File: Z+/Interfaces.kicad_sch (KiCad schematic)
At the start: 13 parts, among them J1 200528-0100, J2 Conn_01x04_MountingPin, J3 USB4110GFA, J4 BG301-06-X-XXXX-X-X_REVC, J5 BG301-06-X-XXXX-X-X_REVC, U1 USBLC6-2P6, U10 USBLC6-2P6

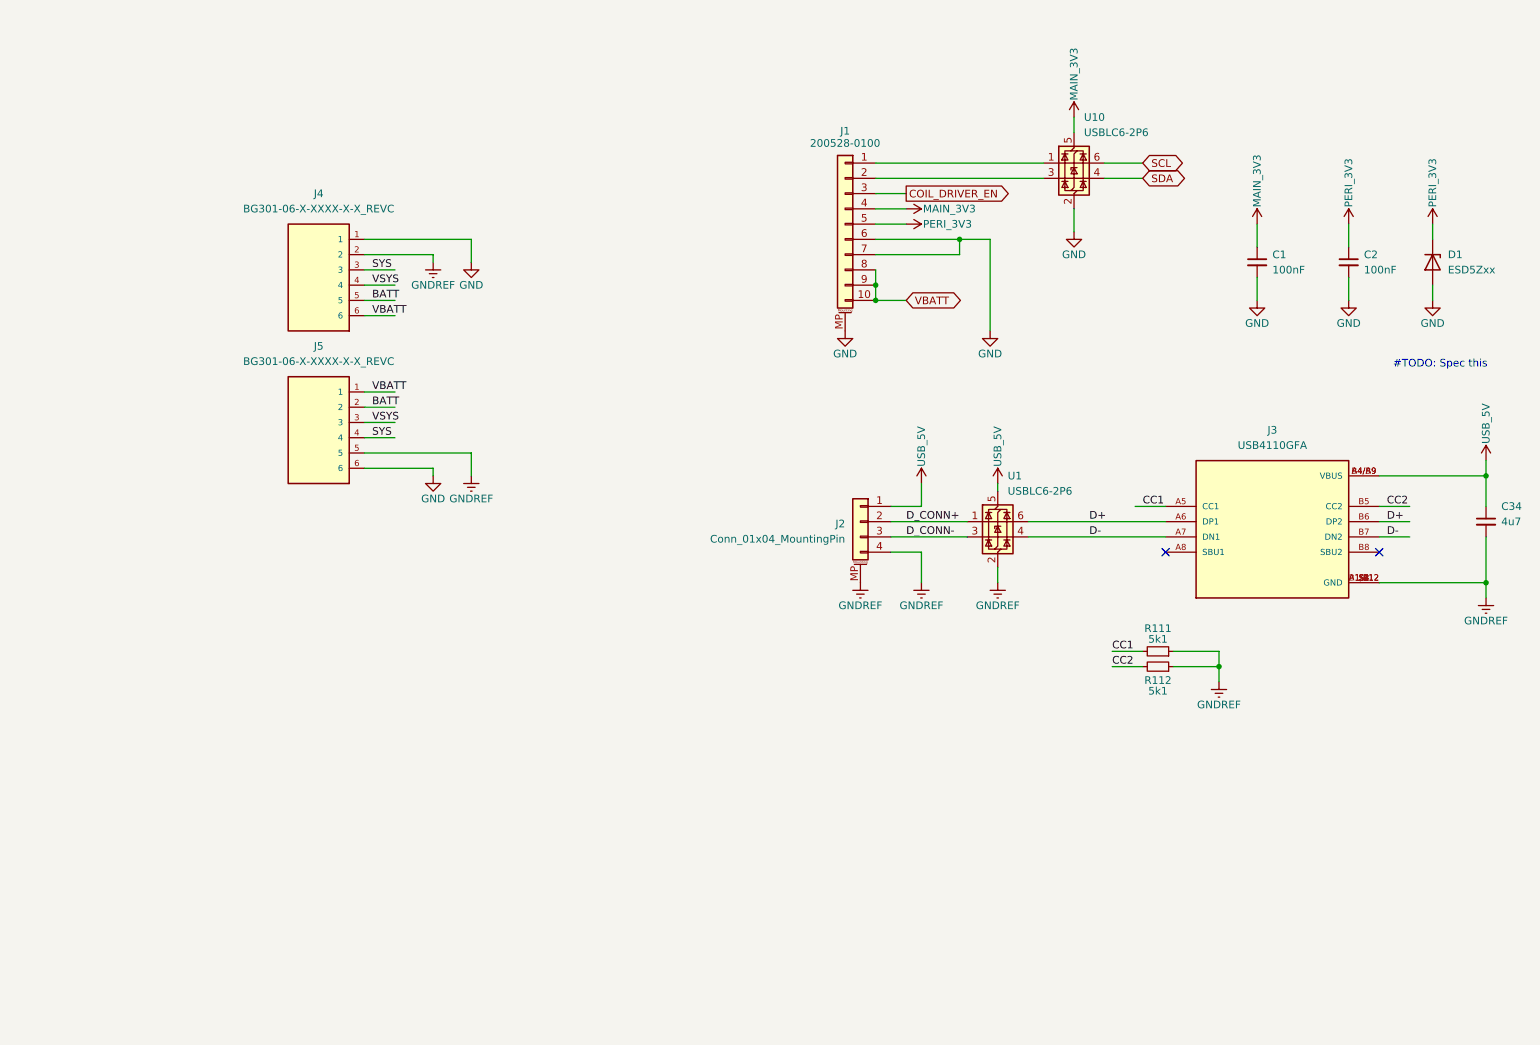
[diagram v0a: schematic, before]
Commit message: More layout work
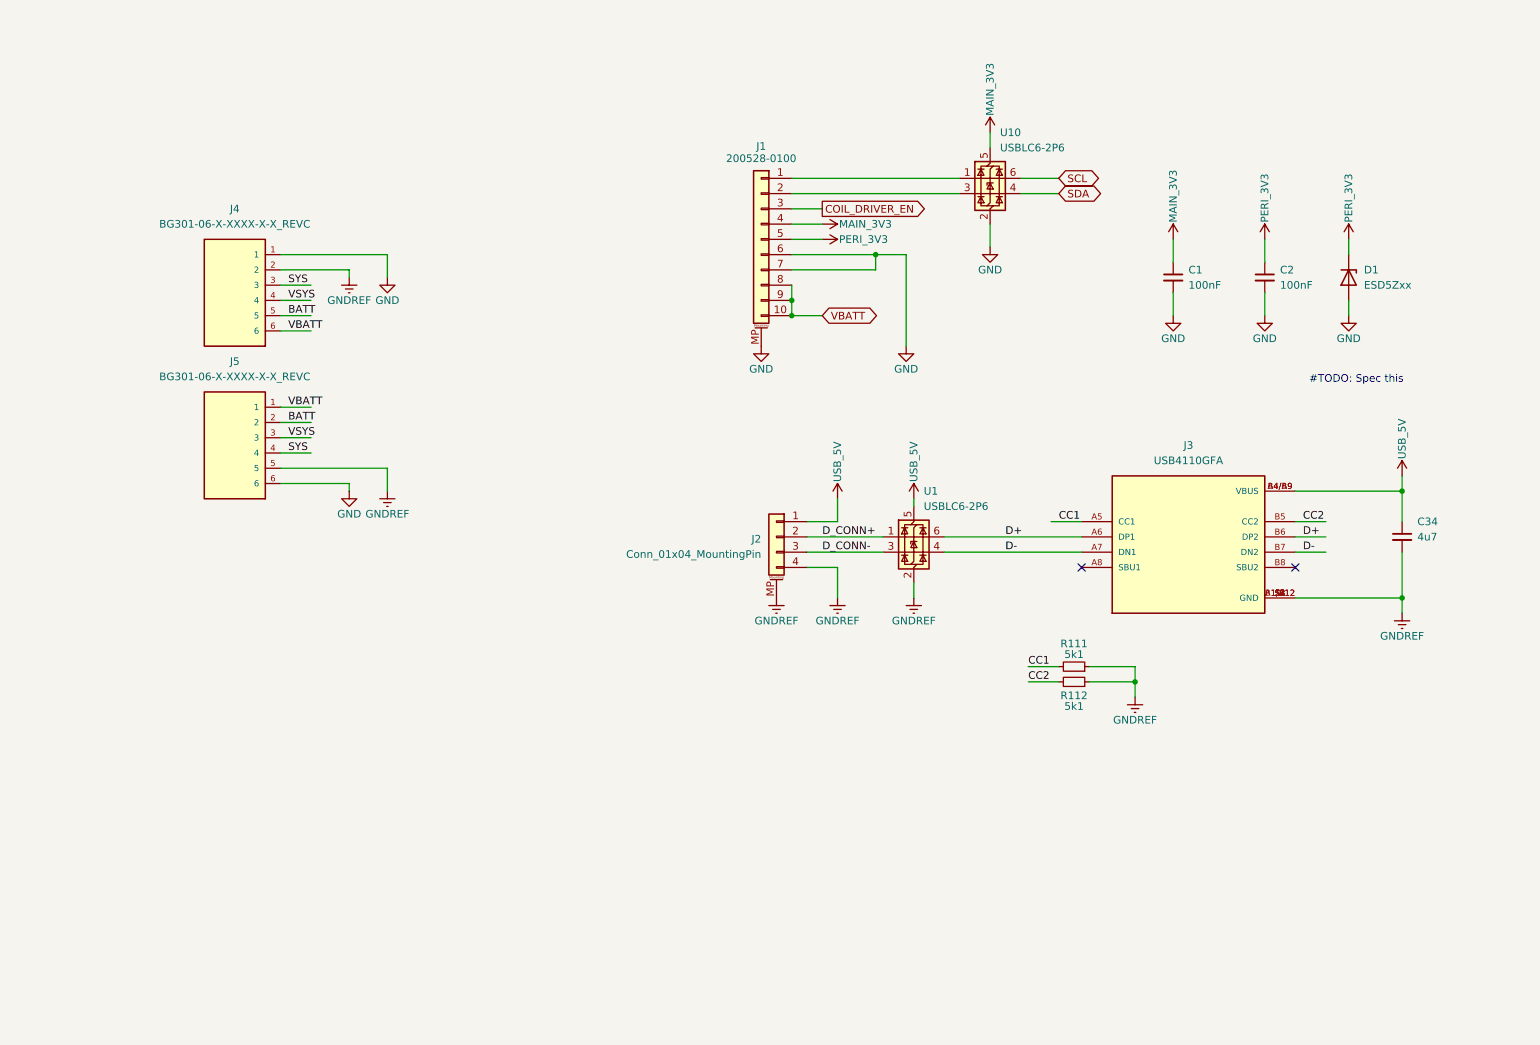
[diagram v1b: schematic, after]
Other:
- moved on the sheet: C1, C2, C34, D1, J1, J2, J3, J4, J5, R111, R112, U1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

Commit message: Finished layout v1
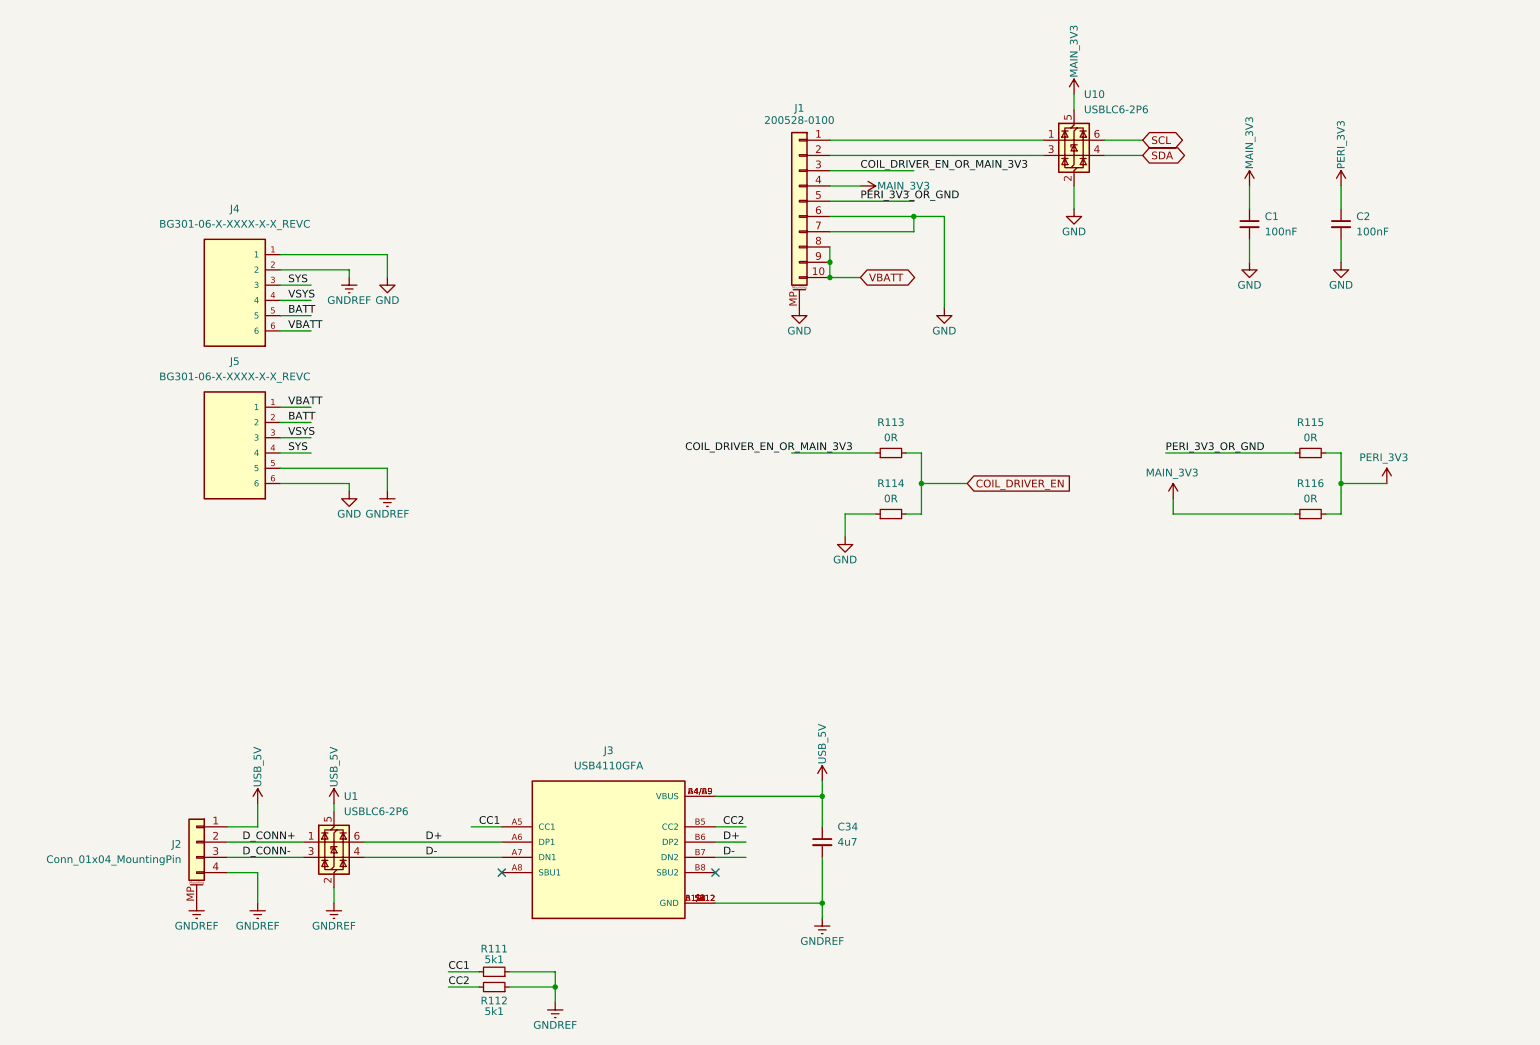
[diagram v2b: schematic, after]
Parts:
- removed D1: ESD5Zxx, Diode_SMD:D_SOD-523, symbol Diode:ESD5Zxx
- added R113, R114, R115, R116: 0R, Resistor_SMD:R_0603_1608Metric, symbol Device:R_Small
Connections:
- net COIL_DRIVER_EN: now also R113.2, R114.2; no longer J1.3 (Pin_3)
- net GND: now also R114.1
- net MAIN_3V3: now also R116.1
- net PERI_3V3: now also R115.2, R116.2; no longer J1.5 (Pin_5)
- new net COIL_DRIVER_EN_OR_MAIN_3V3: J1.3 (Pin_3), R113.1
- new net PERI_3V3_OR_GND: J1.5 (Pin_5), R115.1
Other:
- note removed: "#TODO: Spec this"
- moved on the sheet: C34, J2, J3, R111, R112, U1
